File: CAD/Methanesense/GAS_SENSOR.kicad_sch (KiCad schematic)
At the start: 21 parts, among them Q1 FDS6892A, U2 ADS1115IDGS

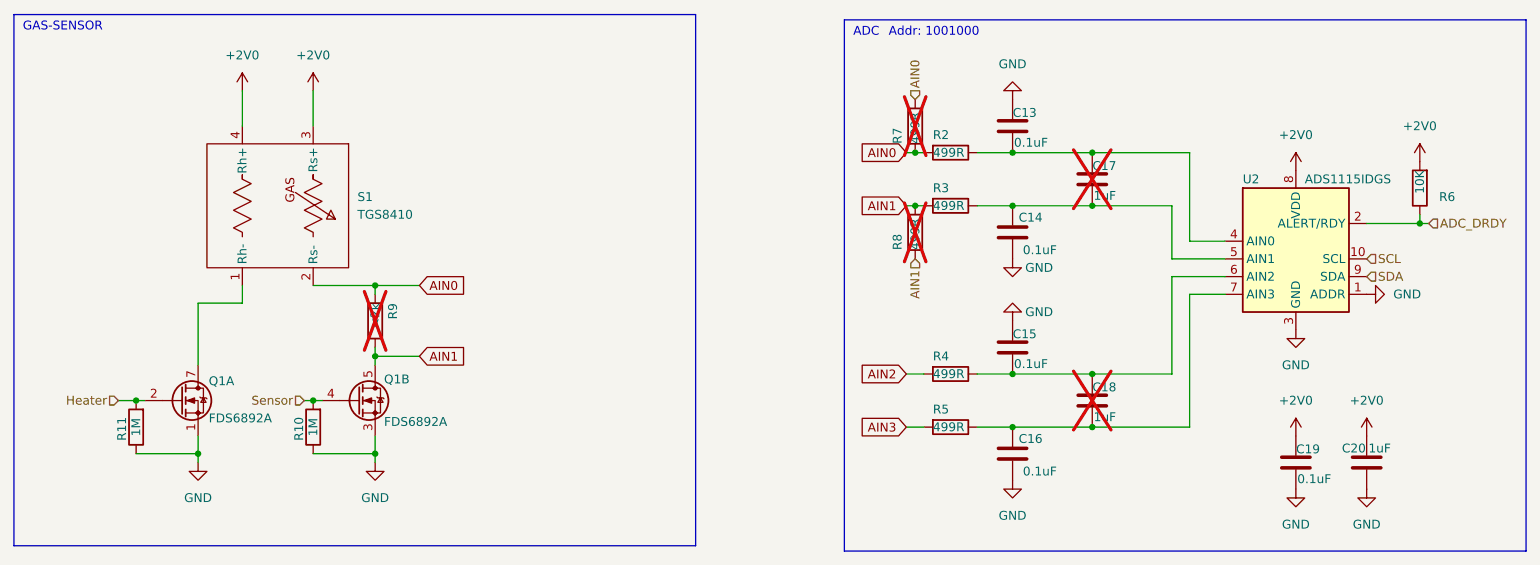
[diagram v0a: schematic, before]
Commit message: Allmost there
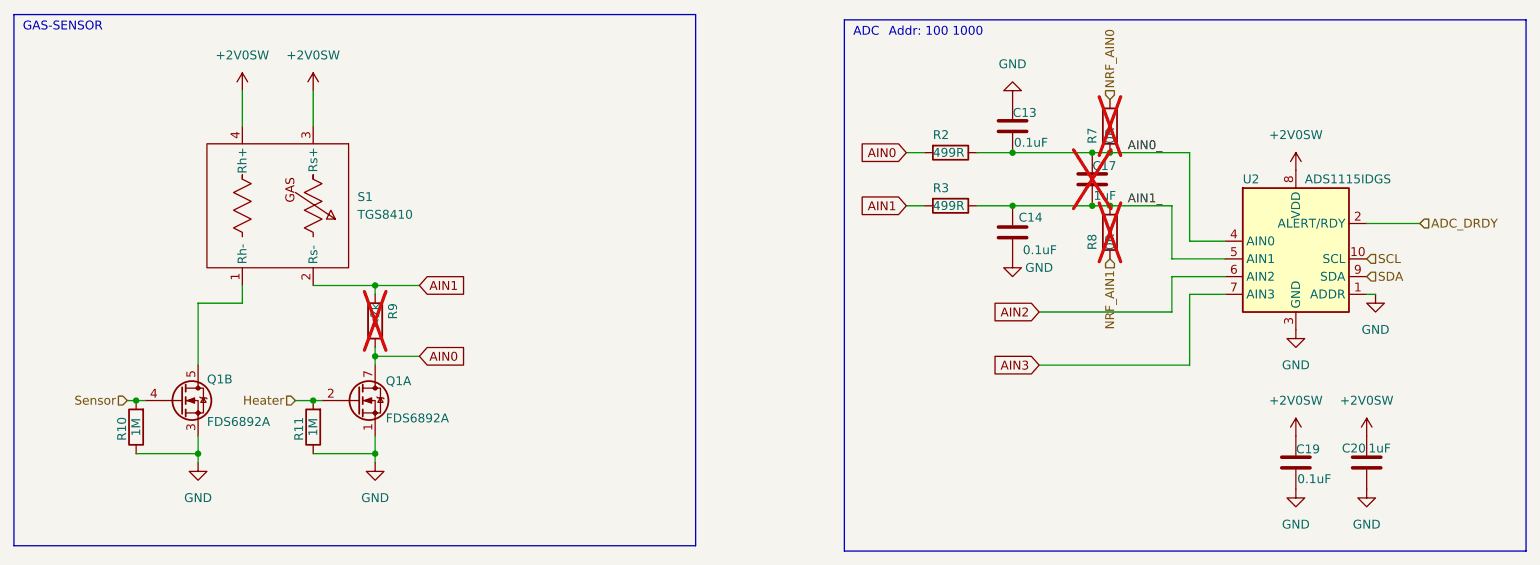
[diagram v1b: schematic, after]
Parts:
- removed C15, C16: 0.1uF, Capacitor_SMD:C_0603_1608Metric, symbol Library:C
- removed C18: 1uF, Capacitor_SMD:C_0603_1608Metric, symbol Library:C
- removed R4, R5: 499R, Resistor_SMD:R_0402_1005Metric, symbol Library:R
- removed R6: 10K, Resistor_SMD:R_0603_1608Metric, symbol Library:R
- R2, R3: footprint Resistor_SMD:R_0402_1005Metric -> Resistor_SMD:R_0603_1608Metric
- R7, R8: value 499R -> 0R; footprint Resistor_SMD:R_0402_1005Metric -> Resistor_SMD:R_0603_1608Metric
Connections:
- net AIN0: now also Q1.7 (D1), Q1.8 (D1), R9.1; no longer R7.1, R7.2, R9.2, S1.2 (Rs-)
- net AIN1: now also R9.2, S1.2 (Rs-); no longer Q1.5 (D2), Q1.6 (D2), R8.1, R8.2, R9.1
- net AIN2: now also U2.6 (AIN2)
- net AIN3: now also U2.7 (AIN3)
- net AIN1_: now reaches C14.2, C17.2, R3.1, U2.5 (AIN1)
- net AIN1_: now also R8.1
- net AIN0_: now reaches C13.2, C17.1, R2.1, U2.4 (AIN0)
- net AIN0_: now also R7.2
- net +2V0 renamed +2V0SW
- new net: Q1.5 (D2), Q1.6 (D2), S1.1 (Rh-)
- new net NRF_AIN0: R7.1
- new net NRF_AIN1: R8.2
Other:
- note added: "Addr: 100 1000"
- note removed: "Addr: 1001000"
- moved on the sheet: Q1A, Q1B, R10, R11, R7, R8

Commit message: WIP
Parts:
- S1: MPN (none) -> TGS8410
- U2: MPN (none) -> ADS1115IDGS
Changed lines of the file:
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@@
+			)
+		)
+		(property "MPN" ""
+			(at 57.15 109.22 0)
+			(effects
+				(font
+					(size 1.27 1.27)
+				)
+				(hide yes)
 			)
 		)
@@
 			)
 		)
+		(property "MPN" ""
+			(at 176.53 85.09 0)
+			(effects
+				(font
+					(size 1.27 1.27)
+				)
+				(hide yes)
+			)
+		)
 		(pin "1"
 		)
@@
 			)
 		)
+		(property "MPN" ""
+			(at 190.5 69.85 0)
+			(effects
+				(font
+					(size 1.27 1.27)
+				)
+				(hide yes)
+			)
+		)
 		(pin "1"
 		)
@@
 					(size 1.27 1.27)
 				)
+			)
+		)
+		(property "MPN" ""
+			(at 82.55 109.22 0)
+			(effects
+				(font
+					(size 1.27 1.27)
+				)
+				(hide yes)
 			)
 		)
@@
 			)
 		)
+		(property "MPN" ""
+			(at 187.96 77.47 0)
+			(effects
+				(font
+					(size 1.27 1.27)
+				)
+				(hide yes)
+			)
+		)
 		(pin "1"
 		)
@@
 			)
 		)
+		(property "MPN" ""
+			(at 217.17 118.11 0)
+			(effects
+				(font
+					(size 1.27 1.27)
+				)
+				(hide yes)
+			)
+		)
 		(pin "1"
 		)
@@
 			)
 		)
+		(property "MPN" ""
+			(at 76.2 113.03 0)
+			(effects
+				(font
+					(size 1.27 1.27)
+				)
+				(hide yes)
+			)
+		)
 		(pin "1"
 		)
@@
 			)
 		)
+		(property "MPN" "ADS1115IDGS"
+			(at 217.17 88.9 0)
+			(effects
+				(font
+					(size 1.27 1.27)
+				)
+				(hide yes)
+			)
+		)
 		(pin "1"
 		)
@@
 					(size 1.27 1.27)
 				)
+			)
+		)
+		(property "MPN" ""
+			(at 167.64 73.66 0)
+			(effects
+				(font
+					(size 1.27 1.27)
+				)
+				(hide yes)
 			)
 		)
@@
 			)
 		)
+		(property "MPN" ""
+			(at 85.09 97.79 0)
+			(effects
+				(font
+					(size 1.27 1.27)
+				)
+				(hide yes)
+			)
+		)
 		(pin "1"
 		)
@@
 			)
 		)
+		(property "MPN" ""
+			(at 227.33 118.11 0)
+			(effects
+				(font
+					(size 1.27 1.27)
+				)
+				(hide yes)
+			)
+		)
 		(pin "1"
 		)
@@
 			)
 		)
+		(property "MPN" ""
+			(at 50.8 113.03 0)
+			(effects
+				(font
+					(size 1.27 1.27)
+				)
+				(hide yes)
+			)
+		)
 		(pin "1"
 		)
@@
 		)
 		(property "LCSC Part #" "C307331"
+			(at 176.53 69.85 0)
+			(effects
+				(font
+					(size 1.27 1.27)
+				)
+				(hide yes)
+			)
+		)
+		(property "MPN" ""
 			(at 176.53 69.85 0)
 			(effects
@@
 			)
 		)
+		(property "MPN" "TGS8410"
+			(at 71.12 81.28 0)
+			(effects
+				(font
+					(size 1.27 1.27)
+				)
+				(hide yes)
+			)
+		)
 		(pin "3"
 		)
@@
 			)
 		)
+		(property "MPN" ""
+			(at 167.64 81.28 0)
+			(effects
+				(font
+					(size 1.27 1.27)
+				)
+				(hide yes)
+			)
+		)
 		(pin "1"
 		)
@@
 			)
 		)
+		(property "MPN" ""
+			(at 190.5 85.09 0)
+			(effects
+				(font
+					(size 1.27 1.27)
+				)
+				(hide yes)
+			)
+		)
